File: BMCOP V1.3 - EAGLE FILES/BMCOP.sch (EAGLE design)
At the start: 18 parts

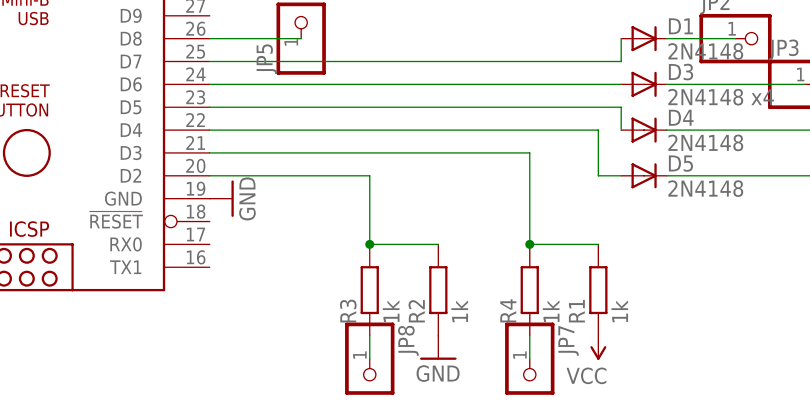
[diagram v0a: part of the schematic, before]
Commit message: Add files via upload
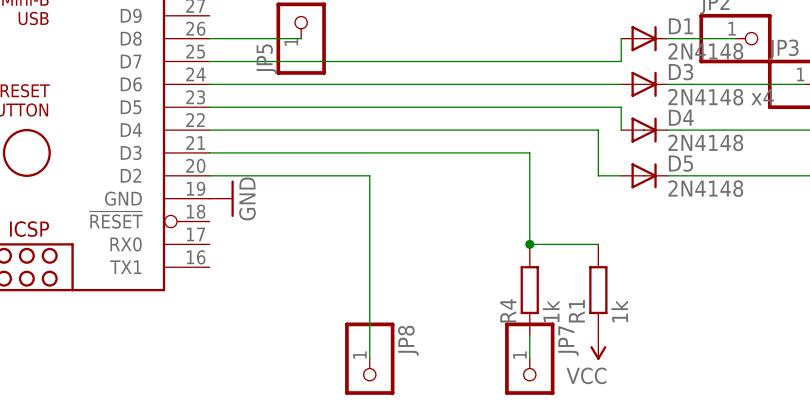
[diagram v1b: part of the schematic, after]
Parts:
- removed R2, R3: 1k, resistor:R-EU_0204/7
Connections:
- removed net N$14: ARDUINO_NANO1.D2, R2.2, R3.2
- net GND: no longer R2.1
- net N$29: now also ARDUINO_NANO1.D2; no longer R3.1
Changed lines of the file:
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@@
 <part name="JP1" library="pinhead_MOD" deviceset="PINHD-1X1" device="" package3d_urn="urn:adsk.eagle:package:22485/2"/>
 <part name="R1" library="resistor" library_urn="urn:adsk.eagle:library:348" deviceset="R-EU_" device="0204/7" package3d_urn="urn:adsk.eagle:package:23498/2" value="1k"/>
-<part name="R2" library="resistor" library_urn="urn:adsk.eagle:library:348" deviceset="R-EU_" device="0204/7" package3d_urn="urn:adsk.eagle:package:23498/2" value="1k"/>
-<part name="R3" library="resistor" library_urn="urn:adsk.eagle:library:348" deviceset="R-EU_" device="0204/7" package3d_urn="urn:adsk.eagle:package:23498/2" value="1k"/>
 <part name="R4" library="resistor" library_urn="urn:adsk.eagle:library:348" deviceset="R-EU_" device="0204/7" package3d_urn="urn:adsk.eagle:package:23498/2" value="1k"/>
 <part name="D1" library="diode" library_urn="urn:adsk.eagle:library:210" deviceset="DIODE-" device="D-7.5" package3d_urn="urn:adsk.eagle:package:43423/1" value="2N4148"/>
@@
 <part name="JP7" library="pinhead_MOD" deviceset="PINHD-1X1" device="" package3d_urn="urn:adsk.eagle:package:22485/2"/>
 <part name="JP8" library="pinhead_MOD" deviceset="PINHD-1X1" device="" package3d_urn="urn:adsk.eagle:package:22485/2"/>
-<part name="GND2" library="supply1" deviceset="GND" device=""/>
 </parts>
 <sheets>
@@
 <attribute name="VALUE" x="292.862" y="-3.81" size="1.778" layer="96" rot="R90"/>
 </instance>
-<instance part="R2" gate="G$1" x="271.78" y="0" smashed="yes" rot="R90">
-<attribute name="NAME" x="270.2814" y="-3.81" size="1.778" layer="95" rot="R90"/>
-<attribute name="VALUE" x="275.082" y="-3.81" size="1.778" layer="96" rot="R90"/>
-</instance>
-<instance part="R3" gate="G$1" x="264.16" y="0" smashed="yes" rot="R90">
-<attribute name="NAME" x="262.6614" y="-3.81" size="1.778" layer="95" rot="R90"/>
-<attribute name="VALUE" x="267.462" y="-3.81" size="1.778" layer="96" rot="R90"/>
-</instance>
 <instance part="R4" gate="G$1" x="281.94" y="0" smashed="yes" rot="R90">
 <attribute name="NAME" x="280.4414" y="-3.81" size="1.778" layer="95" rot="R90"/>
@@
 <attribute name="NAME" x="267.335" y="-3.81" size="1.778" layer="95" rot="R270"/>
 <attribute name="VALUE" x="259.08" y="-3.81" size="1.778" layer="96" rot="R270"/>
-</instance>
-<instance part="GND2" gate="1" x="271.78" y="-7.62" smashed="yes">
-<attribute name="VALUE" x="269.24" y="-10.16" size="1.778" layer="96"/>
 </instance>
 </instances>
@@
 <pinref part="GND7" gate="1" pin="GND"/>
 </segment>
-<segment>
-<pinref part="R2" gate="G$1" pin="1"/>
-<pinref part="GND2" gate="1" pin="GND"/>
-</segment>
 </net>
 <net name="N$1" class="0">
@@
 <pinref part="D5" gate="G$1" pin="C"/>
 <pinref part="JP6" gate="G$1" pin="1"/>
-</segment>
-</net>
-<net name="N$14" class="0">
-<segment>
-<pinref part="ARDUINO_NANO1" gate="G$1" pin="D2"/>
-<wire x1="264.16" y1="12.7" x2="246.38" y2="12.7" width="0.1524" layer="91"/>
-<wire x1="264.16" y1="5.08" x2="264.16" y2="12.7" width="0.1524" layer="91"/>
-<pinref part="R3" gate="G$1" pin="2"/>
-<pinref part="R2" gate="G$1" pin="2"/>
-<wire x1="271.78" y1="5.08" x2="264.16" y2="5.08" width="0.1524" layer="91"/>
-<junction x="264.16" y="5.08"/>
 </segment>
 </net>
@@
 <net name="N$29" class="0">
 <segment>
-<wire x1="264.16" y1="-7.62" x2="264.16" y2="-5.08" width="0.1524" layer="91"/>
-<pinref part="R3" gate="G$1" pin="1"/>
 <pinref part="JP8" gate="G$1" pin="1"/>
-</segment>
-</net>
+<pinref part="ARDUINO_NANO1" gate="G$1" pin="D2"/>
+<wire x1="264.16" y1="12.7" x2="246.38" y2="12.7" width="0.1524" layer="91"/>
+<wire x1="264.16" y1="-7.62" x2="264.16" y2="12.7" width="0.1524" layer="91"/>
+</segment>
+</net>
